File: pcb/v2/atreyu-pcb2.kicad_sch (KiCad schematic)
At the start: 126 parts, among them SW1 SW_Push, SW2 RotaryEncoder_Switch, SW3 RotaryEncoder_Switch, U1 Elite-C

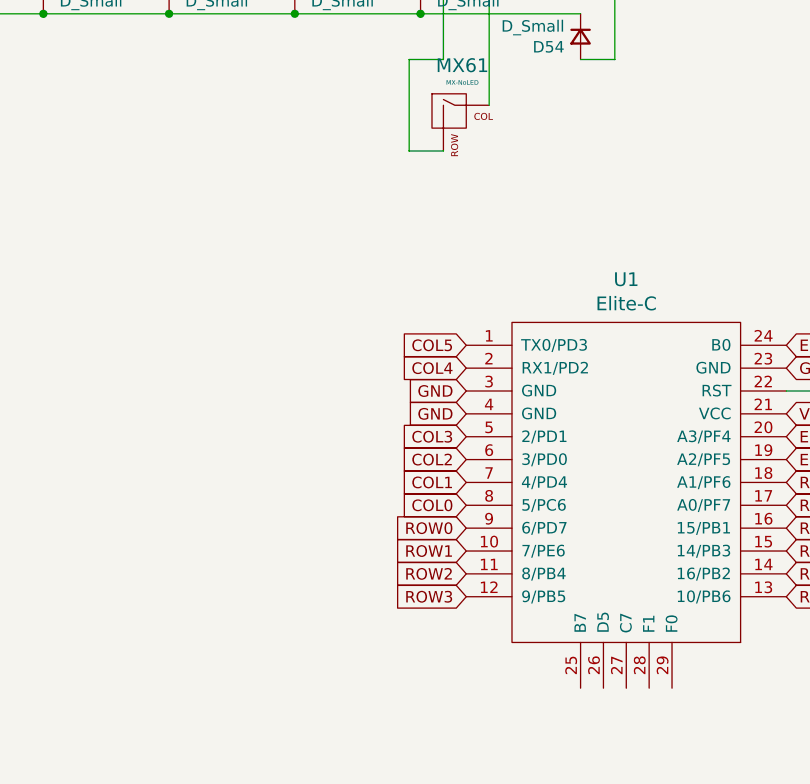
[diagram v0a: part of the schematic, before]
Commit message: Checkpoint commit.
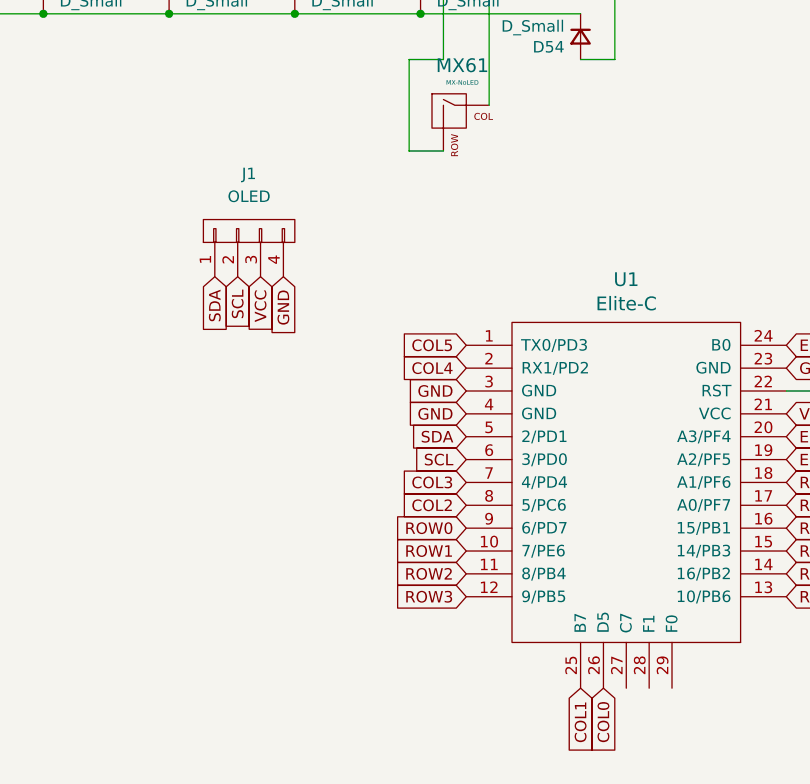
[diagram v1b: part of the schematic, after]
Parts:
- added J1: OLED, Connector_PinHeader_2.54mm:PinHeader_1x04_P2.54mm_Vertical, symbol SouffleKeyboard-rescue:OLED-Lily58-cache
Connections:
- net COL0: now also U1.26 (D5); no longer U1.8 (5/PC6)
- net COL1: now also U1.25 (B7); no longer U1.7 (4/PD4)
- net COL2: now also U1.8 (5/PC6); no longer U1.6 (3/PD0)
- net COL3: now also U1.7 (4/PD4); no longer U1.5 (2/PD1)
- net GND: now also J1.4 (P4)
- net VCC: now also J1.3 (P3)
- new net SCL: J1.2 (P2), U1.6 (3/PD0)
- new net SDA: J1.1 (P1), U1.5 (2/PD1)
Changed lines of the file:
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@@
+    )
+  )
+  (global_label "SCL" (shape input) (at 71.12 140.97 270) (fields_autoplaced)
+    (effects (font (size 1.27 1.27)) (justify right))
+    (property "Intersheet References" "${INTERSHEET_REFS}" (id 0) (at 71.0406 146.8907 90)
+      (effects (font (size 1.27 1.27)) (justify right) hide)
     )
   )
@@
     )
   )
+  (global_label "VCC" (shape input) (at 73.66 140.97 270) (fields_autoplaced)
+    (effects (font (size 1.27 1.27)) (justify right))
+    (property "Intersheet References" "${INTERSHEET_REFS}" (id 0) (at 73.5806 147.0117 90)
+      (effects (font (size 1.27 1.27)) (justify right) hide)
+    )
+  )
+  (global_label "SDA" (shape input) (at 96.52 158.75 180) (fields_autoplaced)
+    (effects (font (size 1.27 1.27)) (justify right))
+    (property "Intersheet References" "${INTERSHEET_REFS}" (id 0) (at 90.5388 158.6706 0)
+      (effects (font (size 1.27 1.27)) (justify right) hide)
+    )
+  )
   (global_label "SW54A" (shape input) (at 190.5 142.24 0) (fields_autoplaced)
     (effects (font (size 1.27 1.27)) (justify left))
@@
     )
   )
-  (global_label "COL3" (shape input) (at 96.52 158.75 180) (fields_autoplaced)
-    (effects (font (size 1.27 1.27)) (justify right))
-    (property "Intersheet References" "${INTERSHEET_REFS}" (id 0) (at 265.43 317.5 0)
+  (global_label "COL3" (shape input) (at 96.52 163.83 180) (fields_autoplaced)
+    (effects (font (size 1.27 1.27)) (justify right))
+    (property "Intersheet References" "${INTERSHEET_REFS}" (id 0) (at 265.43 322.58 0)
       (effects (font (size 1.27 1.27)) hide)
     )
@@
     )
   )
-  (global_label "COL0" (shape input) (at 96.52 166.37 180) (fields_autoplaced)
-    (effects (font (size 1.27 1.27)) (justify right))
-    (property "Intersheet References" "${INTERSHEET_REFS}" (id 0) (at -36.83 17.78 0)
-      (effects (font (size 1.27 1.27)) hide)
-    )
-  )
-  (global_label "COL2" (shape input) (at 96.52 161.29 180) (fields_autoplaced)
-    (effects (font (size 1.27 1.27)) (justify right))
-    (property "Intersheet References" "${INTERSHEET_REFS}" (id 0) (at -36.83 -2.54 0)
+  (global_label "SCL" (shape input) (at 96.52 161.29 180) (fields_autoplaced)
+    (effects (font (size 1.27 1.27)) (justify right))
+    (property "Intersheet References" "${INTERSHEET_REFS}" (id 0) (at 90.5993 161.2106 0)
+      (effects (font (size 1.27 1.27)) (justify right) hide)
+    )
+  )
+  (global_label "COL0" (shape input) (at 111.76 186.69 270) (fields_autoplaced)
+    (effects (font (size 1.27 1.27)) (justify right))
+    (property "Intersheet References" "${INTERSHEET_REFS}" (id 0) (at -36.83 320.04 0)
+      (effects (font (size 1.27 1.27)) hide)
+    )
+  )
+  (global_label "COL2" (shape input) (at 96.52 166.37 180) (fields_autoplaced)
+    (effects (font (size 1.27 1.27)) (justify right))
+    (property "Intersheet References" "${INTERSHEET_REFS}" (id 0) (at -36.83 2.54 0)
       (effects (font (size 1.27 1.27)) hide)
     )
@@
     )
   )
+  (global_label "SDA" (shape input) (at 68.58 140.97 270) (fields_autoplaced)
+    (effects (font (size 1.27 1.27)) (justify right))
+    (property "Intersheet References" "${INTERSHEET_REFS}" (id 0) (at 68.5006 146.9512 90)
+      (effects (font (size 1.27 1.27)) (justify right) hide)
+    )
+  )
   (global_label "COL5" (shape input) (at 96.52 148.59 180) (fields_autoplaced)
     (effects (font (size 1.27 1.27)) (justify right))
@@
     )
   )
-  (global_label "COL1" (shape input) (at 96.52 163.83 180) (fields_autoplaced)
-    (effects (font (size 1.27 1.27)) (justify right))
-    (property "Intersheet References" "${INTERSHEET_REFS}" (id 0) (at -36.83 12.7 0)
+  (global_label "COL1" (shape input) (at 109.22 186.69 270) (fields_autoplaced)
+    (effects (font (size 1.27 1.27)) (justify right))
+    (property "Intersheet References" "${INTERSHEET_REFS}" (id 0) (at -41.91 320.04 0)
       (effects (font (size 1.27 1.27)) hide)
     )
@@
     )
   )
+  (global_label "GND" (shape input) (at 76.2 140.97 270) (fields_autoplaced)
+    (effects (font (size 1.27 1.27)) (justify right))
+    (property "Intersheet References" "${INTERSHEET_REFS}" (id 0) (at 76.1206 147.2536 90)
+      (effects (font (size 1.27 1.27)) (justify right) hide)
+    )
+  )
   (global_label "COL3" (shape input) (at 85.09 26.67 90) (fields_autoplaced)
     (effects (font (size 1.27 1.27)) (justify left))
@@
     (pin "1")
     (pin "2")
+  )
+  (symbol (lib_id "SouffleKeyboard-rescue:OLED-Lily58-cache") (at 72.39 135.89 90) (unit 1)
+    (in_bom yes) (on_board yes)
+    (property "Reference" "J1" (id 0) (at 72.39 129.54 90))
+    (property "Value" "OLED" (id 1) (at 72.39 132.08 90))
+    (property "Footprint" "Connector_PinHeader_2.54mm:PinHeader_1x04_P2.54mm_Vertical" (id 2) (at 73.66 134.62 90)
+      (effects (font (size 1.27 1.27)) hide)
+    )
+    (property "Datasheet" "" (id 3) (at 72.39 135.89 0))
+    (pin "1")
+    (pin "2")
+    (pin "3")
+    (pin "4")
   )
   (symbol (lib_id "Device:D_Small") (at 238.76 91.44 90) (unit 1)
@@
       (reference "D60") (unit 1) (value "D_Small") (footprint "footprints:D3_hybrid_common_hole_connected_fix")
     )
+    (path "/1709f845-7847-4378-aef5-76eaf9944a35"
+      (reference "J1") (unit 1) (value "OLED") (footprint "Connector_PinHeader_2.54mm:PinHeader_1x04_P2.54mm_Vertical")
+    )
     (path "/8a1cdef1-da3d-41b0-8d52-3220205347ba"
